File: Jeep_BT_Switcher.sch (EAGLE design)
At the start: 27 parts, among them J1 MF-CON-2.54mm-01x06, J2 MF-CON-2.54mm-01x04, J3 MF-CON-2.54mm-01x02, U1 AZ4558C, U2 MAX4544CSA+, U3 MAX4544CSA+

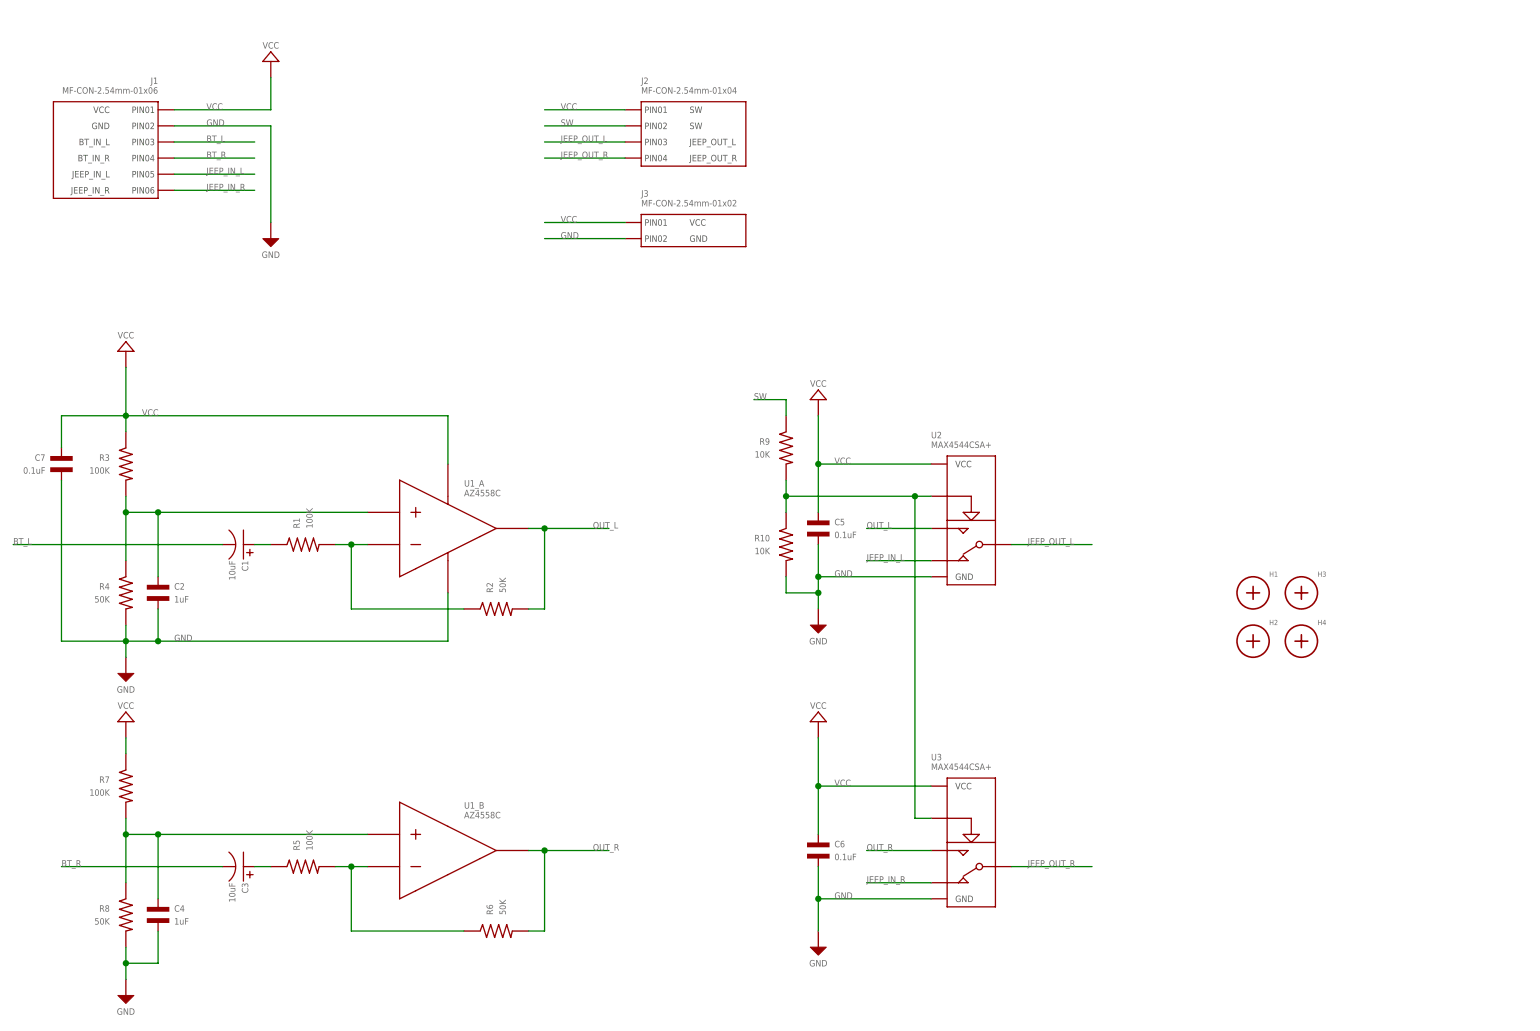
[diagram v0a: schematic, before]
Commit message: Added cam files and XYRS
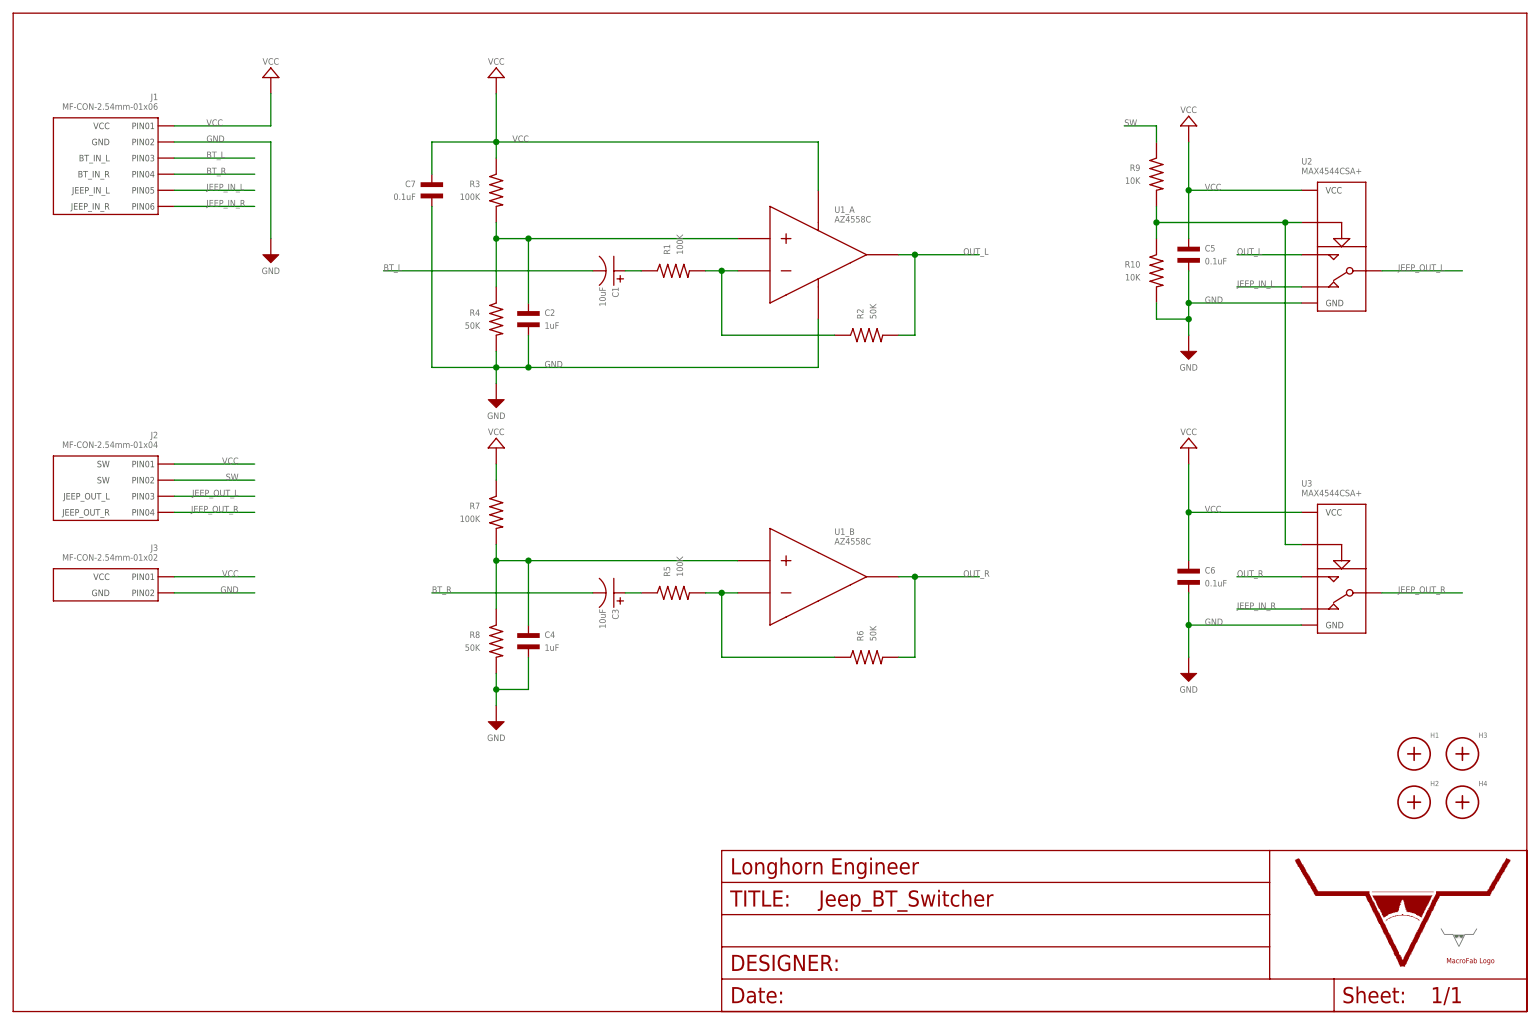
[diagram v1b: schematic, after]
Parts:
- added U$11: LHE_FRAME, PP_Aesthetics:LHE_FRAME
- added U$12: MF_LOGOLOGO_SMALL, PP_Aesthetics:MF_LOGOLOGO_SMALL
- added U$13: LHE_LOGOLHE_LOGO, PP_Aesthetics:LHE_LOGOLHE_LOGO
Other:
- moved on the sheet: C1, C2, C3, C4, C5, C6, C7, H1, H2, H3, H4, J1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
